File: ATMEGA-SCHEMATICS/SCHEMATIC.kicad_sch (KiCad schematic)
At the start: 16 parts, among them U3 ATmega168A, U4 PCF8574N, U5 DS18B20, U6 PCF8574N, Y2 16 MHz

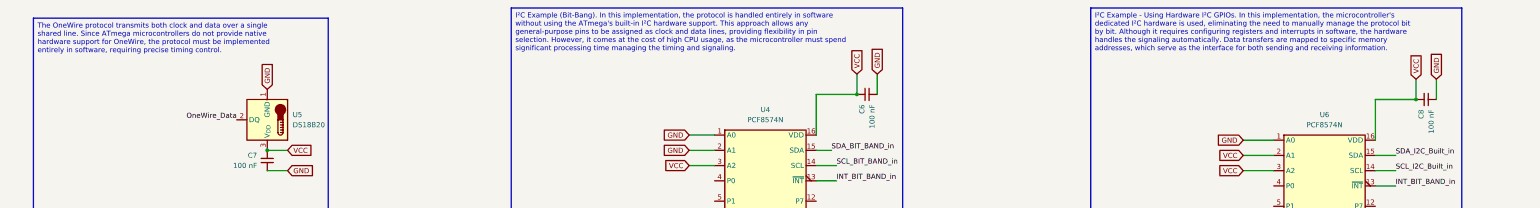
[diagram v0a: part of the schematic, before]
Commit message: .
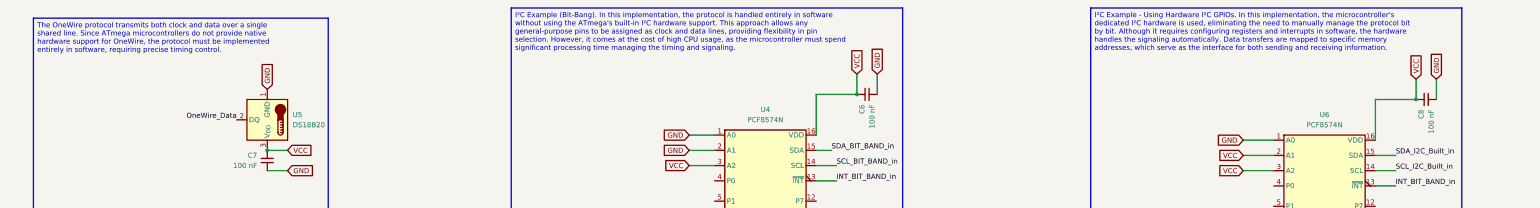
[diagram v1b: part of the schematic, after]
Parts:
- C4, C5, C6, C7, C8: footprint (none) -> Capacitor_THT:CP_Radial_D5.0mm_P2.50mm
- R2, R3, R4, R5, R6, R7: footprint (none) -> Resistor_THT:R_Axial_DIN0207_L6.3mm_D2.5mm_P10.16mm_Horizontal
- U4, U6: footprint (none) -> Package_DIP:CERDIP-16_W7.62mm_SideBrazed_Socket
- Y2: footprint (none) -> Crystal:Resonator-2Pin_W6.0mm_H3.0mm
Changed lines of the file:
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@@
 (kicad_sch
-	(version 20231120)
+	(version 20250114)
 	(generator "eeschema")
-	(generator_version "8.0")
+	(generator_version "9.0")
 	(paper "A3")
+	(text_box "I²C Example - Using Hardware I²C GPIOs. In this implementation, the microcontroller's dedicated I²C hardware is used, eliminating the need to manually manage the protocol bit by bit. Although it requires configuring registers and interrupts in software, the hardware handles the signaling automatically. Data transfers are mapped to specific memory addresses, which serve as the interface for both sending and receiving information."
+		(exclude_from_sim no)
+		(at 280.67 15.24 0)
+		(size 92.71 63.5)
+		(margins 0.9525 0.9525 0.9525 0.9525)
+		(stroke
+			(width 0)
+			(type default)
+		)
+		(fill
+			(type none)
+		)
+		(effects
+			(font
+				(size 1.27 1.27)
+			)
+			(justify left top)
+		)
+	)
+	(text_box "The OneWire protocol transmits both clock and data over a single shared line. Since ATmega microcontrollers do not provide native hardware support for OneWire, the protocol must be implemented entirely in software, requiring precise timing control."
+		(exclude_from_sim no)
+		(at 16.51 17.78 0)
+		(size 73.66 50.8)
+		(margins 0.9525 0.9525 0.9525 0.9525)
+		(stroke
+			(width 0)
+			(type default)
+		)
+		(fill
+			(type none)
+		)
+		(effects
+			(font
+				(size 1.27 1.27)
+			)
+			(justify left top)
+		)
+	)
+	(text_box "I²C Example (Bit-Bang). In this implementation, the protocol is handled entirely in software without using the ATmega's built-in I²C hardware support. This approach allows any general-purpose pins to be assigned as clock and data lines, providing flexibility in pin selection. However, it comes at the cost of high CPU usage, as the microcontroller must spend significant processing time managing the timing and signaling."
+		(exclude_from_sim no)
+		(at 135.89 15.24 0)
+		(size 97.79 62.23)
+		(margins 0.9525 0.9525 0.9525 0.9525)
+		(stroke
+			(width 0)
+			(type default)
+		)
+		(fill
+			(type none)
+		)
+		(effects
+			(font
+				(size 1.27 1.27)
+			)
+			(justify left top)
+		)
+	)
 	(junction
 		(at 361.95 38.1)
@@
 		)
 	)
-	(text_box "I²C Example - Using Hardware I²C GPIOs. In this implementation, the microcontroller's dedicated I²C hardware is used, eliminating the need to manually manage the protocol bit by bit. Although it requires configuring registers and interrupts in software, the hardware handles the signaling automatically. Data transfers are mapped to specific memory addresses, which serve as the interface for both sending and receiving information."
-		(exclude_from_sim no)
-		(at 280.67 15.24 0)
-		(size 92.71 63.5)
-		(stroke
-			(width 0)
-			(type default)
-		)
-		(fill
-			(type none)
-		)
-		(effects
-			(font
-				(size 1.27 1.27)
-			)
-			(justify left top)
-		)
-	)
-	(text_box "The OneWire protocol transmits both clock and data over a single shared line. Since ATmega microcontrollers do not provide native hardware support for OneWire, the protocol must be implemented entirely in software, requiring precise timing control."
-		(exclude_from_sim no)
-		(at 16.51 17.78 0)
-		(size 73.66 50.8)
-		(stroke
-			(width 0)
-			(type default)
-		)
-		(fill
-			(type none)
-		)
-		(effects
-			(font
-				(size 1.27 1.27)
-			)
-			(justify left top)
-		)
-	)
-	(text_box "I²C Example (Bit-Bang). In this implementation, the protocol is handled entirely in software without using the ATmega's built-in I²C hardware support. This approach allows any general-purpose pins to be assigned as clock and data lines, providing flexibility in pin selection. However, it comes at the cost of high CPU usage, as the microcontroller must spend significant processing time managing the timing and signaling."
-		(exclude_from_sim no)
-		(at 135.89 15.24 0)
-		(size 97.79 62.23)
-		(stroke
-			(width 0)
-			(type default)
-		)
-		(fill
-			(type none)
-		)
-		(effects
-			(font
-				(size 1.27 1.27)
-			)
-			(justify left top)
-		)
-	)
 	(label "SDA_BIT_BAND_in"
 		(at 132.08 123.19 0)
-		(fields_autoplaced yes)
 		(effects
 			(font
@@
 	(label "INT_BIT_BAND_in"
 		(at 356.87 59.69 0)
-		(fields_autoplaced yes)
 		(effects
 			(font
@@
 	(label "SDA_I2C_Built_in"
 		(at 119.38 105.41 0)
-		(fields_autoplaced yes)
 		(effects
 			(font
@@
 	(label "SCL_I2C_Built_in"
 		(at 100.33 115.57 0)
-		(fields_autoplaced yes)
 		(effects
 			(font
@@
 	(label "SCL_BIT_BAND_in"
 		(at 123.19 115.57 0)
-		(fields_autoplaced yes)
 		(effects
 			(font
@@
 	(label "RXD_Built_in"
 		(at 25.4 120.65 180)
-		(fields_autoplaced yes)
 		(effects
 			(font
@@
 	(label "INT_BIT_BAND_in"
 		(at 217.17 58.42 0)
-		(fields_autoplaced yes)
 		(effects
 			(font
@@
 	(label "SCL_I2C_Built_in"
 		(at 356.87 55.88 0)
-		(fields_autoplaced yes)
 		(effects
 			(font
@@
 	(label "SDA_BIT_BAND_in"
 		(at 215.9 50.8 0)
-		(fields_autoplaced yes)
 		(effects
 			(font
@@
 	(label "TXD_Built_in"
 		(at 25.4 125.73 180)
-		(fields_autoplaced yes)
 		(effects
 			(font
@@
 	(label "INT_BIT_BAND_in"
 		(at 139.7 129.54 0)
-		(fields_autoplaced yes)
 		(effects
 			(font
@@
 	(label "OneWire_Data"
 		(at 41.91 135.89 180)
-		(fields_autoplaced yes)
 		(effects
 			(font
@@
 	(label "SCL_BIT_BAND_in"
 		(at 217.17 54.61 0)
-		(fields_autoplaced yes)
 		(effects
 			(font
@@
 	(label "SDA_I2C_Built_in"
 		(at 356.87 52.07 0)
-		(fields_autoplaced yes)
 		(effects
 			(font
@@
 	(label "OneWire_Data"
 		(at 67.31 43.18 180)
-		(fields_autoplaced yes)
 		(effects
 			(font
@@
 			)
 		)
-		(property "Footprint" ""
+		(property "Footprint" "Capacitor_THT:CP_Radial_D5.0mm_P2.50mm"
 			(at 224.79 36.83 0)
 			(effects
@@
 			)
 		)
-		(property "Footprint" ""
+		(property "Footprint" "Resistor_THT:R_Axial_DIN0207_L6.3mm_D2.5mm_P10.16mm_Horizontal"
 			(at 92.202 111.76 90)
 			(effects
@@
 			)
 		)
-		(property "Footprint" ""
+		(property "Footprint" "Crystal:Resonator-2Pin_W6.0mm_H3.0mm"
 			(at 36.83 158.75 0)
 			(effects
@@
 			)
 		)
-		(property "Footprint" ""
+		(property "Footprint" "Capacitor_THT:CP_Radial_D5.0mm_P2.50mm"
 			(at 364.49 38.1 0)
 			(effects
@@
 			)
 		)
-		(property "Footprint" ""
+		(property "Footprint" "Capacitor_THT:CP_Radial_D5.0mm_P2.50mm"
 			(at 74.93 53.34 0)
 			(effects
@@
 			)
 		)
-		(property "Footprint" ""
+		(property "Footprint" "Resistor_THT:R_Axial_DIN0207_L6.3mm_D2.5mm_P10.16mm_Horizontal"
 			(at 123.19 113.538 90)
 			(effects
@@
 			)
 		)
-		(property "Footprint" ""
+		(property "Footprint" "Resistor_THT:R_Axial_DIN0207_L6.3mm_D2.5mm_P10.16mm_Horizontal"
 			(at 50.038 132.08 90)
 			(effects
@@
 			)
 		)
-		(property "Footprint" ""
+		(property "Footprint" "Resistor_THT:R_Axial_DIN0207_L6.3mm_D2.5mm_P10.16mm_Horizontal"
 			(at 143.51 130.302 90)
 			(effects
@@
 			)
 		)
-		(property "Footprint" ""
+		(property "Footprint" "Capacitor_THT:CP_Radial_D5.0mm_P2.50mm"
 			(at 30.48 162.56 0)
 			(effects
@@
 			)
 		)
-		(property "Footprint" ""
+		(property "Footprint" "Resistor_THT:R_Axial_DIN0207_L6.3mm_D2.5mm_P10.16mm_Horizontal"
 			(at 135.89 123.952 90)
 			(effects
@@
 			)
 		)
-		(property "Footprint" ""
+		(property "Footprint" "Capacitor_THT:CP_Radial_D5.0mm_P2.50mm"
 			(at 30.48 154.94 0)
 			(effects
@@
 			)
 		)
-		(property "Footprint" ""
+		(property "Footprint" "Resistor_THT:R_Axial_DIN0207_L6.3mm_D2.5mm_P10.16mm_Horizontal"
 			(at 127 116.332 90)
 			(effects
@@
 			)
 		)
-		(property "Footprint" ""
+		(property "Footprint" "Package_DIP:CERDIP-16_W7.62mm_SideBrazed_Socket"
 			(at 339.09 62.23 0)
 			(effects
@@
 			)
 		)
-		(property "Footprint" ""
+		(property "Footprint" "Package_DIP:CERDIP-16_W7.62mm_SideBrazed_Socket"
 			(at 199.39 60.96 0)
 			(effects
